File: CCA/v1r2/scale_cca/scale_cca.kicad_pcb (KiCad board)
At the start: 2 copper layers, 22.2 x 57.5 mm, 27 parts

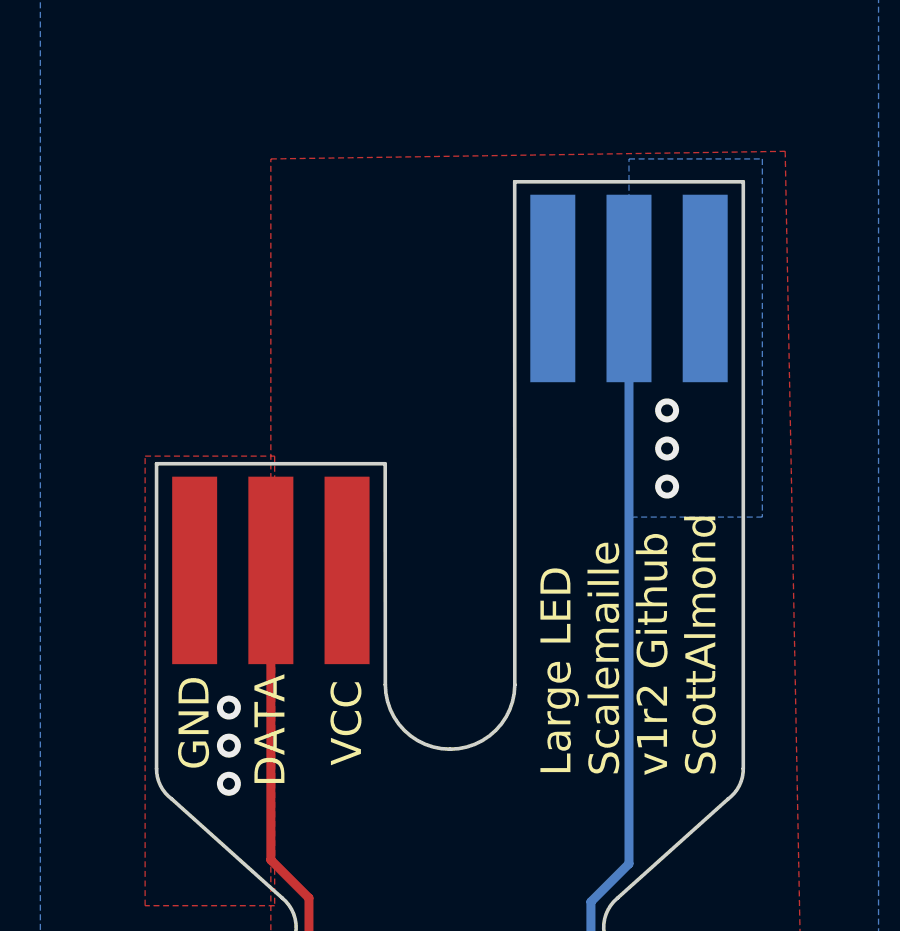
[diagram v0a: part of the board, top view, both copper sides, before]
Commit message: pdf mock up
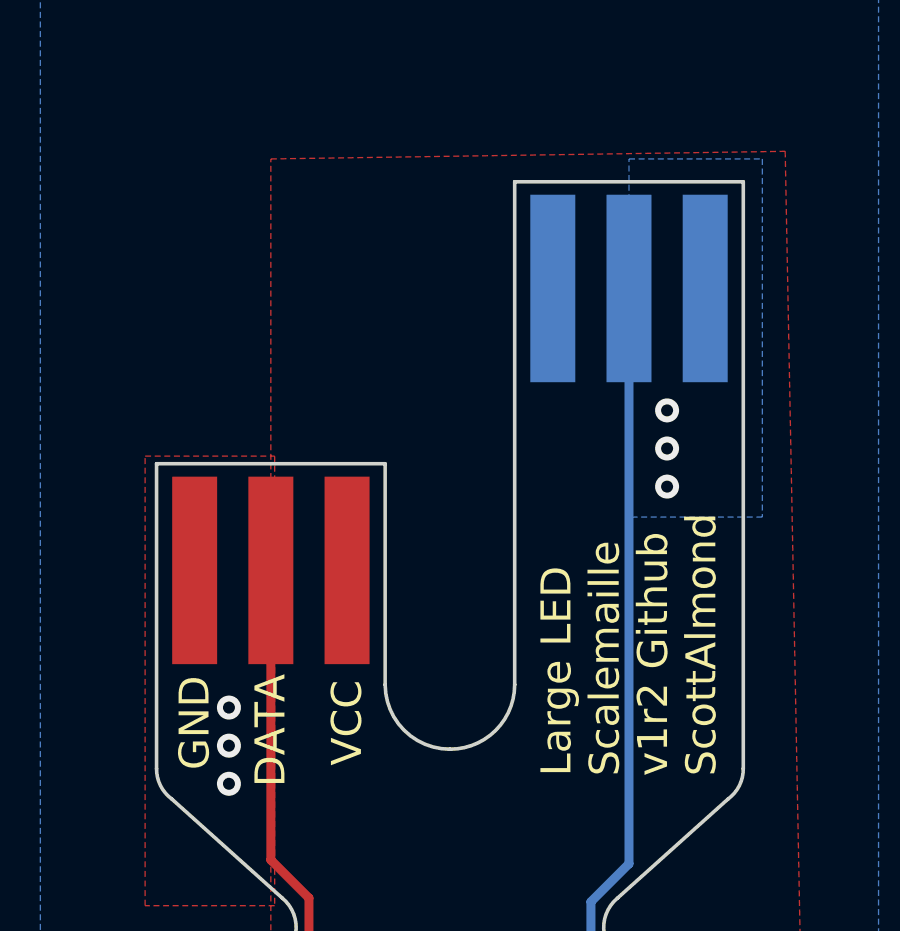
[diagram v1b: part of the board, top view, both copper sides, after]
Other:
- board text added: "7.11 mm"
- board text added: "7.62 mm"
- board text added: "Stiffiner BOTTOM"
- board text added: "Stiffiner TOP"
- board text removed: "BOTTOM PAD"
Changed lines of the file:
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@@
     (property "Sheetfile" "scale_cca.kicad_sch")
     (property "Sheetname" "")
-    (fp_text reference "TP4" (at 5.08 0 90 unlocked) (layer "Dwgs.User")
+    (fp_text reference "TP4" (at 1.778 0 90 unlocked) (layer "Dwgs.User")
       (effects (font (size 1 1) (thickness 0.15)))
     )
@@
     (property "Sheetfile" "scale_cca.kicad_sch")
     (property "Sheetname" "")
-    (fp_text reference "TP5" (at 5.08 0 90 unlocked) (layer "Dwgs.User")
+    (fp_text reference "TP5" (at 1.778 0 90 unlocked) (layer "Dwgs.User")
       (effects (font (size 1 1) (thickness 0.15)))
     )
@@
     (property "Sheetfile" "scale_cca.kicad_sch")
     (property "Sheetname" "")
-    (fp_text reference "TP2" (at 5.08 0 90 unlocked) (layer "Dwgs.User")
+    (fp_text reference "TP2" (at 1.778 0 90 unlocked) (layer "Dwgs.User")
       (effects (font (size 1 1) (thickness 0.15)))
     )
@@
     (property "Sheetfile" "scale_cca.kicad_sch")
     (property "Sheetname" "")
-    (fp_text reference "TP1" (at -5.08 0 90 unlocked) (layer "Dwgs.User")
+    (fp_text reference "TP1" (at -1.778 0 90 unlocked) (layer "Dwgs.User")
       (effects (font (size 1 1) (thickness 0.15)))
     )
@@
     (property "Sheetfile" "scale_cca.kicad_sch")
     (property "Sheetname" "")
-    (fp_text reference "TP6" (at -5.08 0 90 unlocked) (layer "Dwgs.User")
+    (fp_text reference "TP6" (at -1.778 0 90 unlocked) (layer "Dwgs.User")
       (effects (font (size 1 1) (thickness 0.15)))
     )
@@
     (property "Sheetfile" "scale_cca.kicad_sch")
     (property "Sheetname" "")
-    (fp_text reference "TP3" (at 5.08 0 90 unlocked) (layer "Dwgs.User")
+    (fp_text reference "TP3" (at 1.778 0 90 unlocked) (layer "Dwgs.User")
       (effects (font (size 1 1) (thickness 0.15)))
     )
@@
       (net 3 "VCC") (pinfunction "1") (pintype "passive"))
   )
+  (gr_line (start 25.4635 20.193) (end 25.9715 19.685) (layer "Dwgs.User") (width 0.2))
   (gr_arc (start 45.734539 43.307001) (end 36.5125 26.67) (angle -122) (layer "Dwgs.User") (width 0.12))
+  (gr_line (start 37.5285 3.683) (end 38.0365 4.191) (layer "Dwgs.User") (width 0.2))
+  (gr_line (start 46.4185 2.667) (end 45.9105 3.175) (layer "Dwgs.User") (width 0.2))
+  (gr_line (start 34.417 12.065) (end 33.909 11.557) (layer "Dwgs.User") (width 0.2))
+  (gr_line (start 46.4185 2.667) (end 45.9105 2.159) (layer "Dwgs.User") (width 0.2))
+  (gr_line (start 25.4635 20.193) (end 25.4635 13.081) (layer "Dwgs.User") (width 0.2))
+  (gr_line (start 25.4635 13.081) (end 24.9555 13.589) (layer "Dwgs.User") (width 0.2))
+  (gr_line (start 46.4185 2.667) (end 38.9255 2.667) (layer "Dwgs.User") (width 0.2))
+  (gr_line (start 25.4635 13.081) (end 25.9715 13.589) (layer "Dwgs.User") (width 0.2))
   (gr_line (start 50.8 43.18) (end 50.8 43.18) (layer "Dwgs.User") (width 0.12))
+  (gr_line (start 38.7985 2.667) (end 39.3065 3.175) (layer "Dwgs.User") (width 0.2))
   (gr_arc (start 27.290461 43.306999) (end 36.5125 26.67) (angle 122) (layer "Dwgs.User") (width 0.12))
   (gr_rect (start 26.7335 13.081) (end 34.3535 20.193) (layer "Dwgs.User") (width 0.2) (fill none))
+  (gr_line (start 26.797 12.065) (end 27.305 11.557) (layer "Dwgs.User") (width 0.2))
   (gr_line (start 22.86 43.307) (end 50.8 43.307) (layer "Dwgs.User") (width 0.12))
+  (gr_line (start 37.5285 10.795) (end 37.5285 3.683) (layer "Dwgs.User") (width 0.2))
   (gr_line (start 36.5125 22.86) (end 36.5125 63.5) (layer "Dwgs.User") (width 0.12))
+  (gr_line (start 26.797 12.065) (end 27.305 12.573) (layer "Dwgs.User") (width 0.2))
   (gr_line (start 31.0125 29.337) (end 42.0125 29.337) (layer "Dwgs.User") (width 0.12))
+  (gr_line (start 37.5285 3.683) (end 37.0205 4.191) (layer "Dwgs.User") (width 0.2))
+  (gr_line (start 34.417 12.065) (end 26.924 12.065) (layer "Dwgs.User") (width 0.2))
+  (gr_line (start 37.5285 10.795) (end 37.0205 10.287) (layer "Dwgs.User") (width 0.2))
   (gr_circle (center 36.5125 33.3) (end 41.2075 33.3) (layer "Dwgs.User") (width 0.12) (fill none))
   (gr_circle (center 36.5125 33.30001) (end 42.2275 33.30001) (layer "Dwgs.User") (width 0.12) (fill none))
+  (gr_line (start 25.4635 20.193) (end 24.9555 19.685) (layer "Dwgs.User") (width 0.2))
   (gr_arc (start 45.382143 43.307) (end 36.5125 25.4) (angle -127.3) (layer "Dwgs.User") (width 0.12))
   (gr_arc (start 27.392857 43.307) (end 36.2625 25.4) (angle 127.3) (layer "Dwgs.User") (width 0.12))
   (gr_line (start 25.4 60.964) (end 47.625 60.964) (layer "Dwgs.User") (width 0.12))
   (gr_arc (start 45.632143 43.307) (end 36.7625 25.4) (angle -127.3) (layer "Dwgs.User") (width 0.12))
+  (gr_line (start 38.7985 2.667) (end 39.3065 2.159) (layer "Dwgs.User") (width 0.2))
+  (gr_line (start 37.5285 10.795) (end 38.0365 10.287) (layer "Dwgs.User") (width 0.2))
+  (gr_line (start 34.417 12.065) (end 33.909 12.573) (layer "Dwgs.User") (width 0.2))
+  (gr_rect (start 38.6715 3.683) (end 46.2915 10.795) (layer "Dwgs.User") (width 0.2) (fill none))
   (gr_rect (start 25.4 25.4) (end 47.625 61.214) (layer "Dwgs.User") (width 0.12) (fill none))
   (gr_line (start 42.1005 27.558999) (end 45.7835 24.257) (layer "Edge.Cuts") (width 0.12))
@@
   (gr_arc (start 42.901749 28.53575) (end 42.1005 27.558999) (angle -90) (layer "Edge.Cuts") (width 0.12))
   (gr_line (start 26.7335 13.081) (end 26.7335 23.241) (layer "Edge.Cuts") (width 0.12))
-  (gr_arc (start 36.511461 20.444816) (end 34.359758 20.445853) (angle -90) (layer "Edge.Cuts") (width 0.12))
+  (gr_arc (start 36.511456 20.43855) (end 34.3535 20.445853) (angle -89.83376508) (layer "Edge.Cuts") (width 0.12))
   (gr_arc (start 30.12325 28.535748) (end 31.1 29.337) (angle -90) (layer "Edge.Cuts") (width 0.12))
   (gr_line (start 46.2915 3.683) (end 46.2915 23.241) (layer "Edge.Cuts") (width 0.12))
   (gr_arc (start 45.04904 23.254769) (end 45.7835 24.257) (angle -54.4) (layer "Edge.Cuts") (width 0.12))
-  (gr_arc (start 36.519435 20.439313) (end 36.5125 22.596516) (angle -90) (layer "Edge.Cuts") (width 0.12))
+  (gr_arc (start 36.519417 20.444443) (end 36.5125 22.596516) (angle -90.13612571) (layer "Edge.Cuts") (width 0.12))
   (gr_line (start 30.9245 27.558999) (end 27.2415 24.257) (layer "Edge.Cuts") (width 0.12))
   (gr_arc (start 27.975221 23.255139) (end 27.2415 24.257) (angle 54.43489273) (layer "Edge.Cuts") (width 0.12))
   (gr_line (start 26.7335 13.081) (end 34.3535 13.081) (layer "Edge.Cuts") (width 0.12))
   (gr_circle (center 36.5125 33.30001) (end 40.9575 33.30001) (layer "Edge.Cuts") (width 0.12) (fill none) (locked))
-  (gr_line (start 38.6715 3.683) (end 38.676637 20.446247) (layer "Edge.Cuts") (width 0.12))
-  (gr_line (start 34.3535 13.081) (end 34.359758 20.445853) (layer "Edge.Cuts") (width 0.12))
+  (gr_line (start 38.6715 3.683) (end 38.6715 20.446247) (layer "Edge.Cuts") (width 0.12))
+  (gr_line (start 34.3535 13.081) (end 34.3535 20.445853) (layer "Edge.Cuts") (width 0.12))
   (gr_line (start 38.6715 3.683) (end 46.2915 3.683) (layer "Edge.Cuts") (width 0.12))
   (gr_arc (start 27.638752 43.309294) (end 41.925 29.337) (angle 108) (layer "Edge.Cuts") (width 0.12))
@@
     (effects (font (size 1 1) (thickness 0.15)) (justify left))
   )
-  (gr_text "BOTTOM\nPAD" (at 23.6855 16.129 90) (layer "Dwgs.User")
-    (effects (font (size 1.5 1.5) (thickness 0.15)))
+  (gr_text "7.62 mm" (at 34.0995 10.541) (layer "Dwgs.User")
+    (effects (font (size 1 1) (thickness 0.15)) (justify right))
+  )
+  (gr_text "7.11 mm" (at 35.8775 3.937 90) (layer "Dwgs.User")
+    (effects (font (size 1 1) (thickness 0.15)) (justify right))
+  )
+  (gr_text "7.11 mm" (at 23.8125 13.335 90) (layer "Dwgs.User")
+    (effects (font (size 1 1) (thickness 0.15)) (justify right))
+  )
+  (gr_text "7.62 mm" (at 45.9105 1.143) (layer "Dwgs.User")
+    (effects (font (size 1 1) (thickness 0.15)) (justify right))
+  )
+  (gr_text "Stiffiner\nBOTTOM" (at 26.0985 11.049) (layer "Dwgs.User")
+    (effects (font (size 1 1) (thickness 0.15)) (justify right))
   )
   (gr_text "#PCBWAY#" (at 36.5125 28.067) (layer "Dwgs.User")
     (effects (font (size 0.762 0.762) (thickness 0.15)))
   )
+  (gr_text "Stiffiner\nTOP" (at 38.0365 1.397) (layer "Dwgs.User")
+    (effects (font (size 1 1) (thickness 0.15)) (justify right))
+  )
   (segment (start 28.184489 44.904011) (end 30.5435 42.545) (width 0.5) (layer "F.Cu") (net 1))
